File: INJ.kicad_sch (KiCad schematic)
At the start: 10 parts, among them U1 VNLD5160TR-E, U2 VNLD5160TR-E

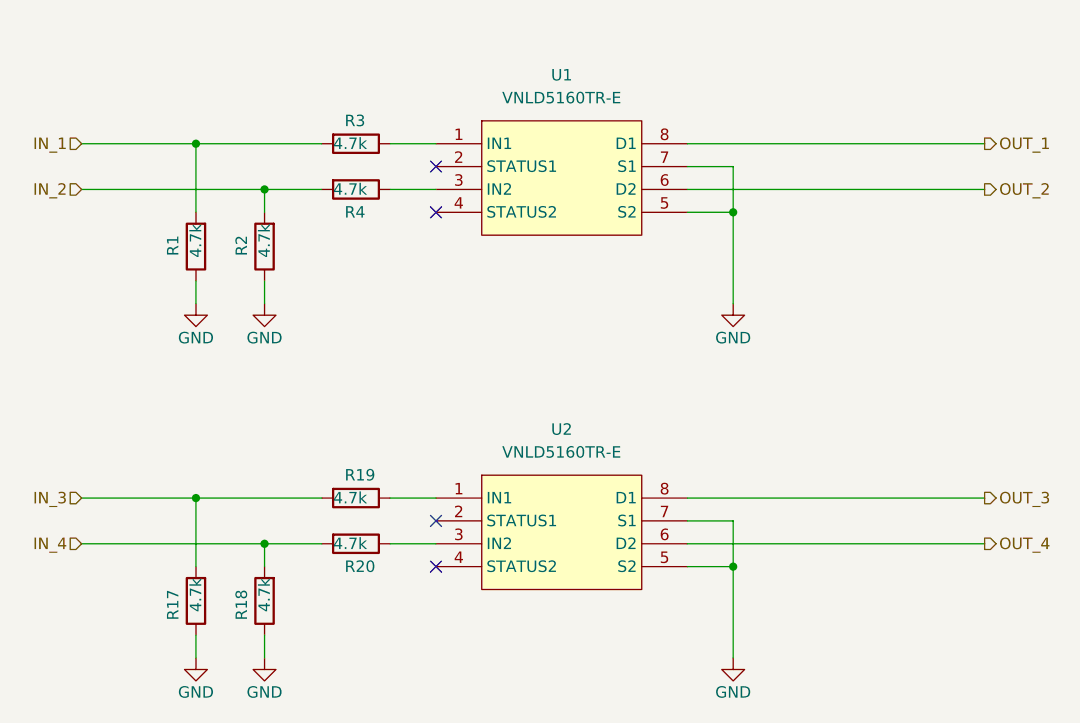
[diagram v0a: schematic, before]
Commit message: Rev G
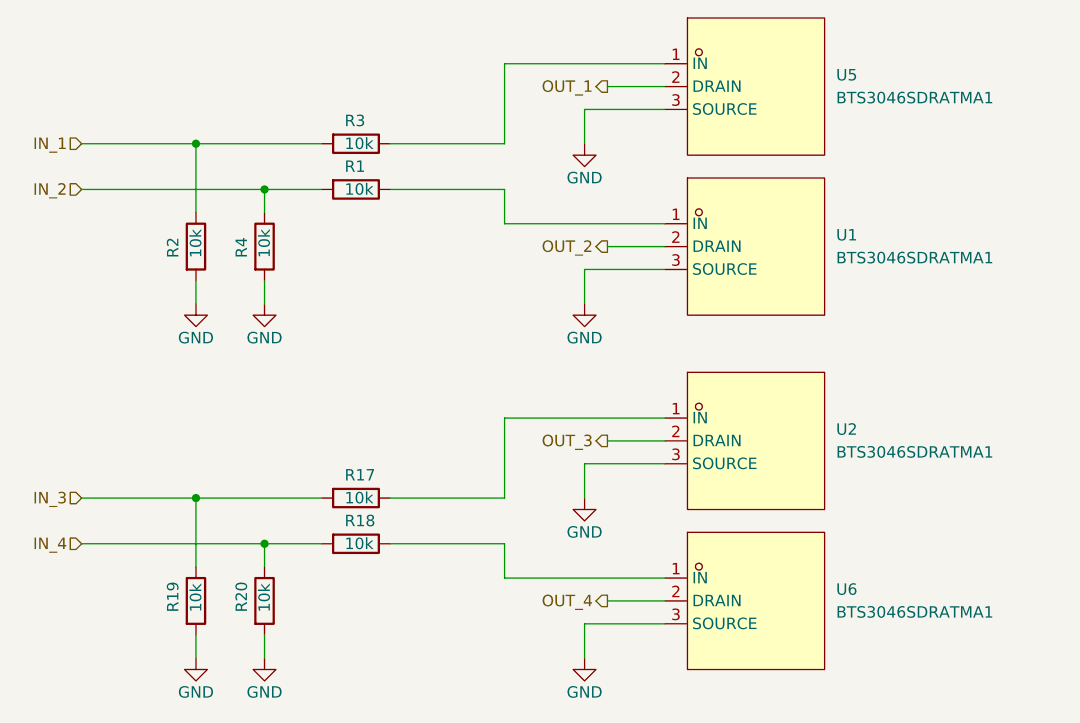
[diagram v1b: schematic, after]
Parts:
- removed U1, U2: VNLD5160TR-E, Package_SO:SOIC-8_3.9x4.9mm_P1.27mm, symbol chips:VNLD5160
- added U1, U2, U5, U6: BTS3046SDRATMA1, easyeda2kicad:PG-TO252-3_L6.5-W6.2-P4.57-LS10.0-BR-CW-1, symbol easyeda2kicad:BTS3046SDRATMA1
- R1, R17, R18, R19, R2, R20, R3, R4: value 4.7k -> 10k; LCSC C23162 -> C98220
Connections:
- net GND: now also R19.2, R2.2, R20.2, R4.2, U1.3 (SOURCE), U2.3 (SOURCE), U5.3 (SOURCE), U6.3 (SOURCE); no longer R1.1, R17.1, R18.1, R2.1
- net IN_1: now also R2.1; no longer R1.2
- net IN_2: now also R1.2, R4.1; no longer R2.2, R4.2
- net IN_3: now also R19.1; no longer R19.2
- net IN_4: now also R20.1; no longer R20.2
- net OUT_1: now also U5.2 (DRAIN)
- net OUT_2: now also U1.2 (DRAIN)
- net OUT_3: now also U2.2 (DRAIN)
- net OUT_4: now also U6.2 (DRAIN)
- net at R3.1: now also U5.1 (IN)
- new net: R1.1, U1.1 (IN)
- new net: R18.1, U6.1 (IN)
- new net: R17.1, U2.1 (IN)
- no-connect marks 4 -> 0
